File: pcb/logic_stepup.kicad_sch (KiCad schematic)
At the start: 8 parts, among them U21 74LVC138

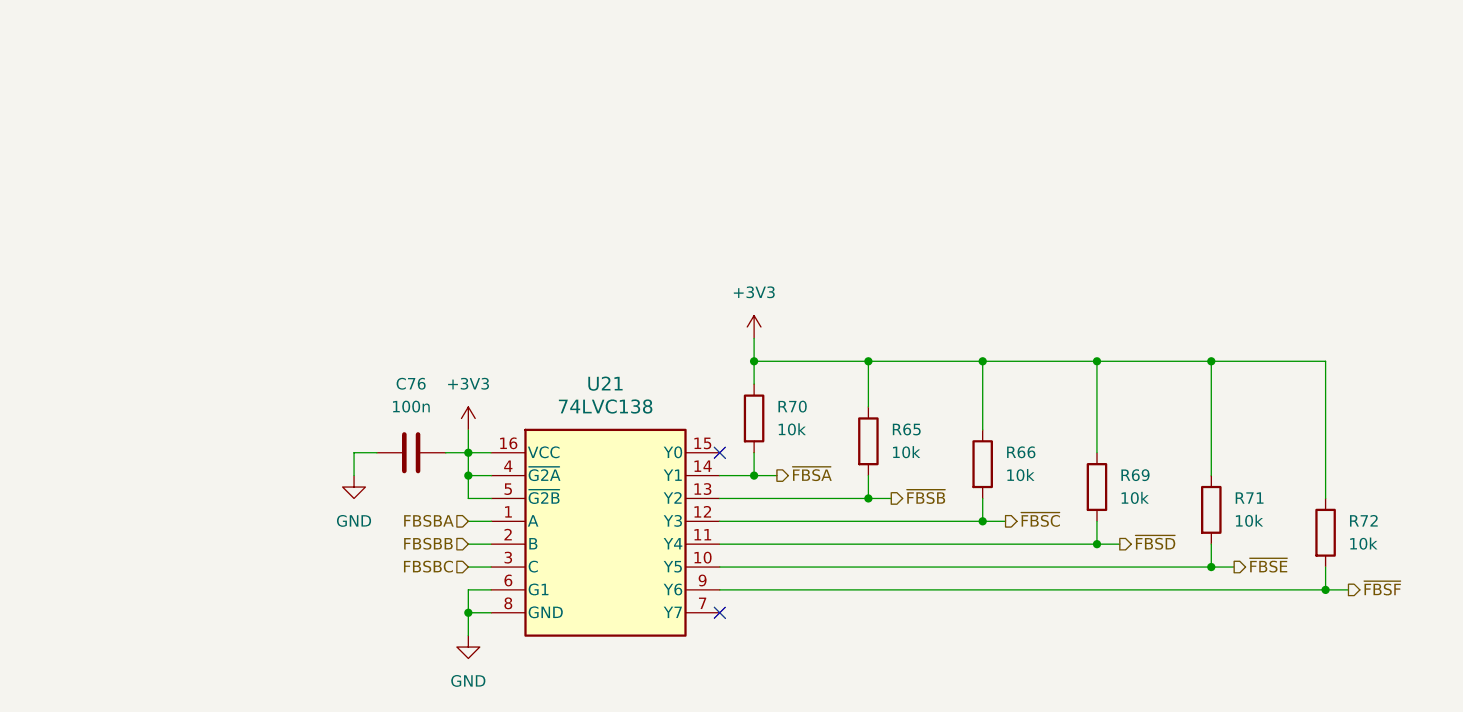
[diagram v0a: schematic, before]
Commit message: chore: many changes checkpoint
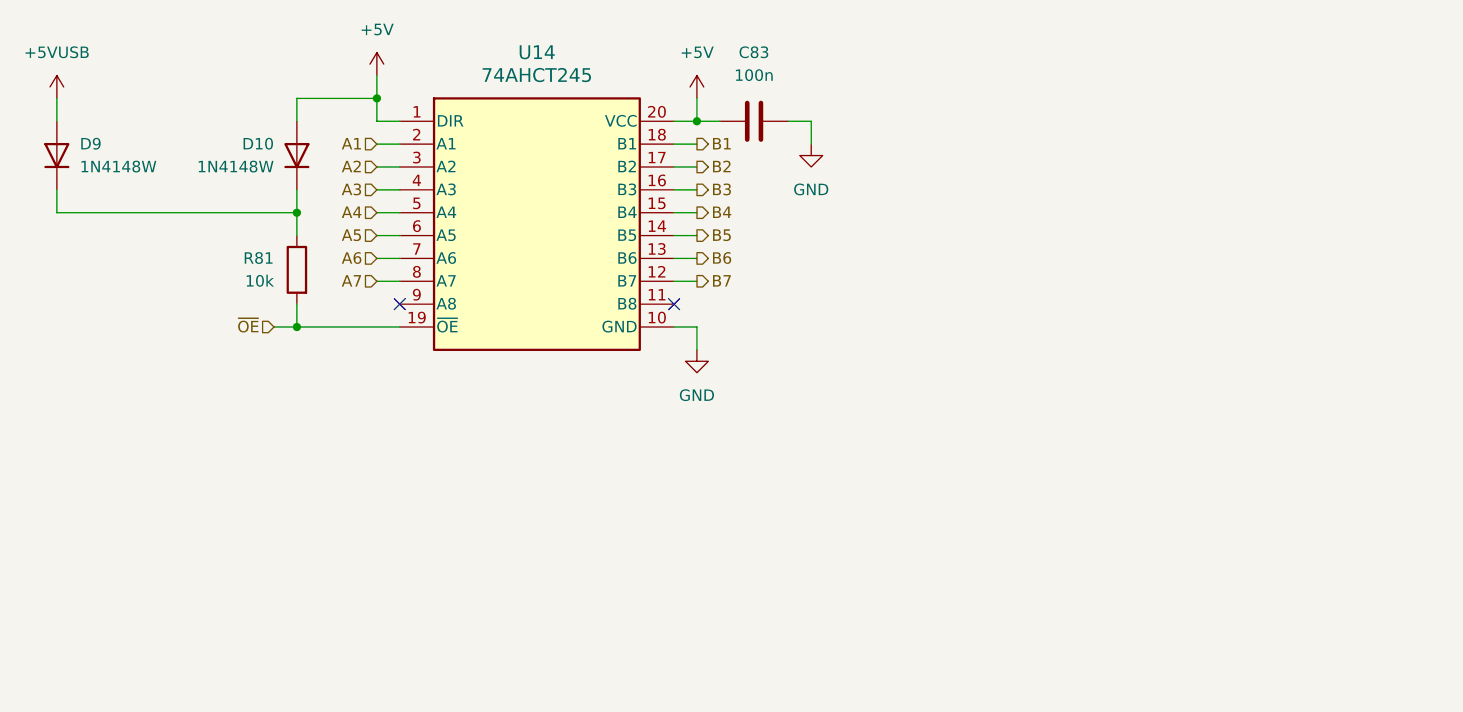
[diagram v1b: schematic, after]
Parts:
- removed C76: 100n, Capacitor_SMD:C_0603_1608Metric, symbol Device:C
- removed R65, R66, R69, R70, R71, R72: 10k, Resistor_SMD:R_0603_1608Metric, symbol Device:R
- removed U21: 74LVC138, Package_SO:TSSOP-16_4.4x5mm_P0.65mm, symbol project_library:74LVC138
- added C83: 100n, Capacitor_SMD:C_0603_1608Metric, symbol Device:C
- added D10, D9: 1N4148W, Diode_SMD:D_SOD-123, symbol Diode:1N4148W
- added R81: 10k, Resistor_SMD:R_0603_1608Metric, symbol Device:R
- added U14: 74AHCT245, Package_SO:SSOP-20_5.3x7.2mm_P0.65mm, symbol project_library:74AHCT245
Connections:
- net GND: now also C83.2, U14.10 (GND)
- new net: D10.1 (K), D9.1 (K), R81.1
- new net +5V: C83.1, D10.2 (A), U14.1 (DIR), U14.20 (VCC)
- new net +5VUSB: D9.2 (A)
- new net A1: U14.2 (A1)
- new net A2: U14.3 (A2)
- new net A3: U14.4 (A3)
- new net A4: U14.5 (A4)
- new net A5: U14.6 (A5)
- new net A6: U14.7 (A6)
- new net A7: U14.8 (A7)
- new net B1: U14.18 (B1)
- new net B2: U14.17 (B2)
- new net B3: U14.16 (B3)
- new net B4: U14.15 (B4)
- new net B5: U14.14 (B5)
- new net B6: U14.13 (B6)
- new net B7: U14.12 (B7)
- new net ~{OE}: R81.2, U14.19 (~{OE})
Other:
- company: (none) -> WRJT
- title: (none) -> 3V3 to 5V logic step-up
